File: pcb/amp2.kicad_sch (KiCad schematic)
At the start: 25 parts, among them Q3 BFP640, Q4 BFP640

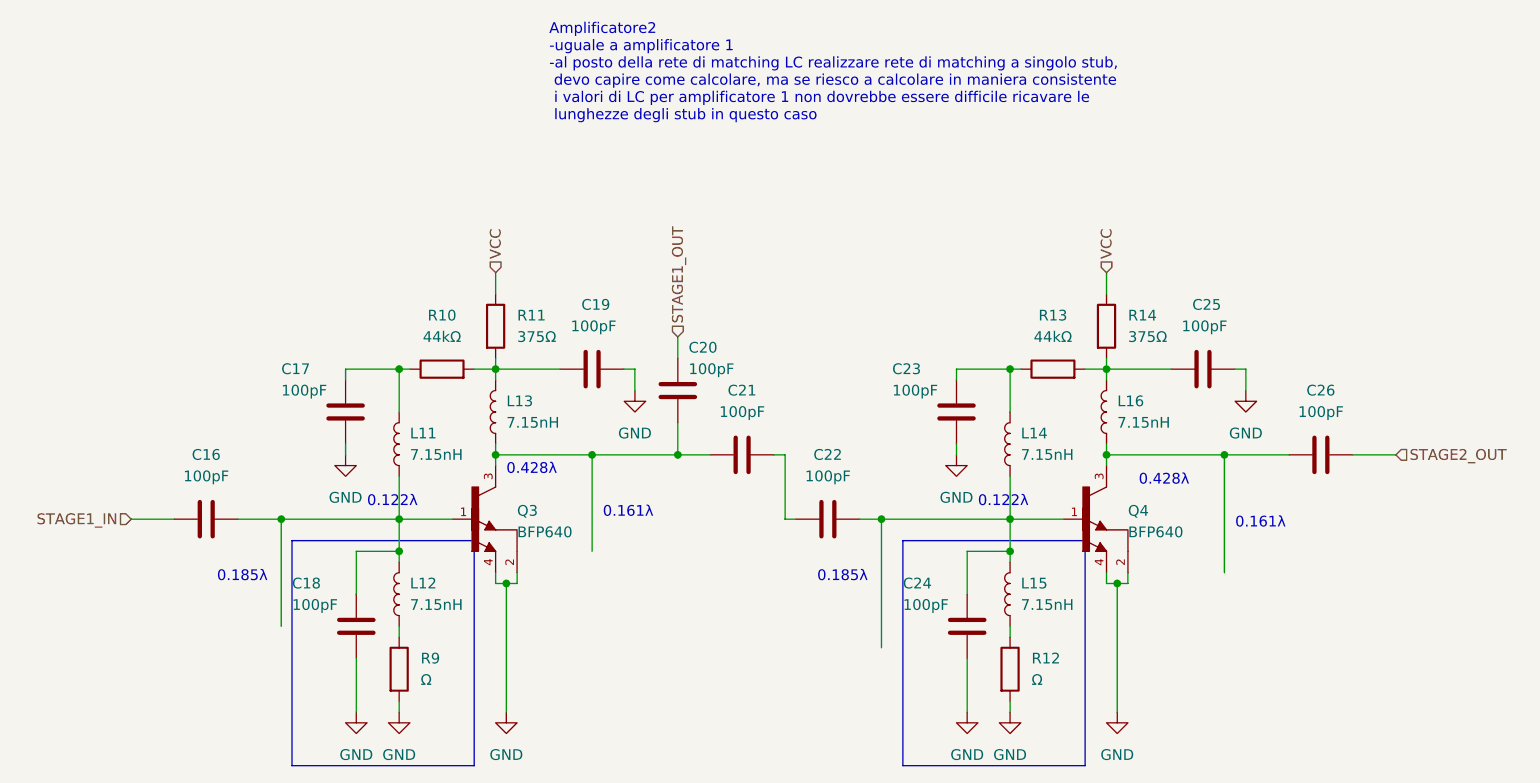
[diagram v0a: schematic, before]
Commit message: Schematic modified as discussed
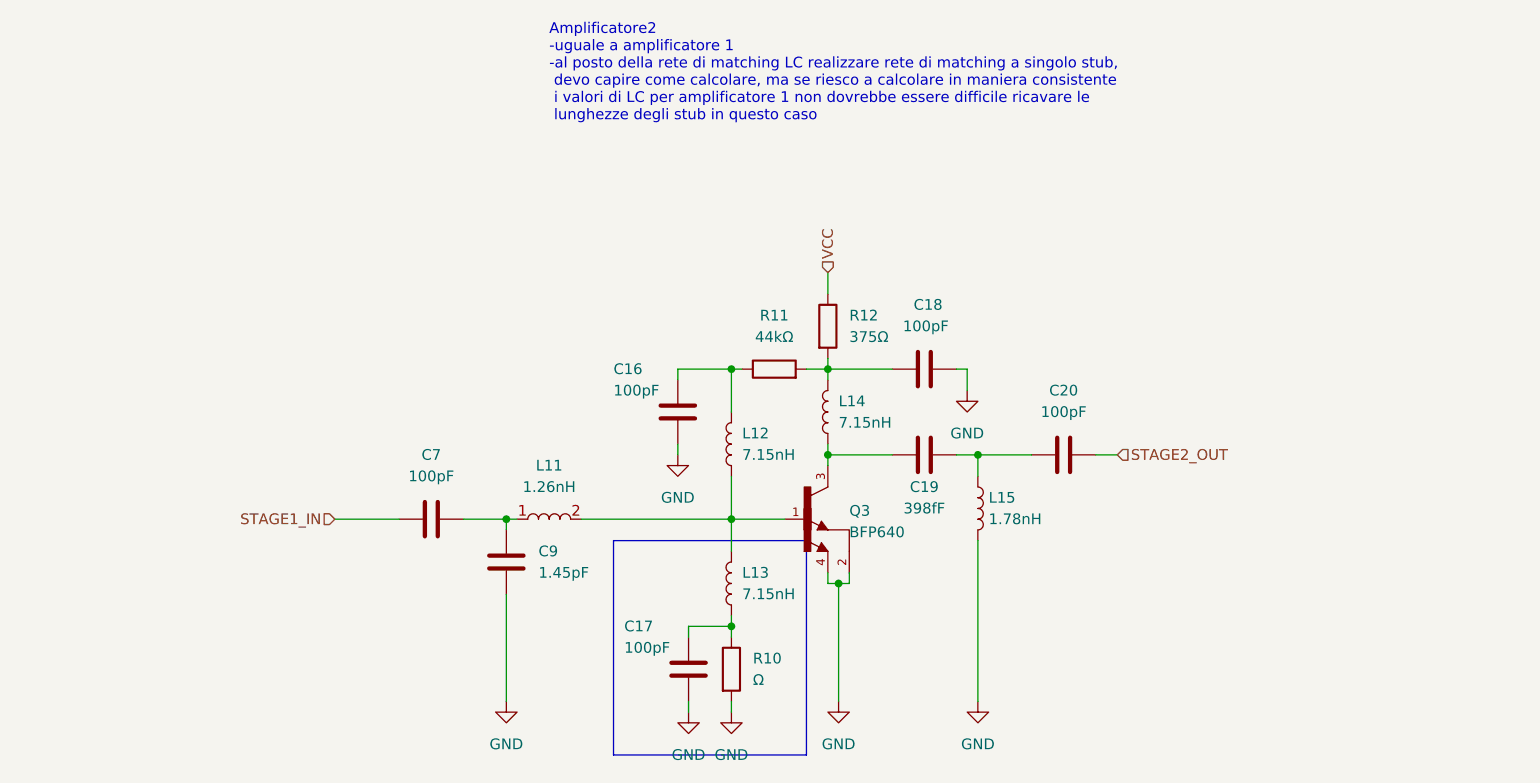
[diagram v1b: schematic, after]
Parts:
- removed C21, C22, C23, C24, C25, C26: 100pF, symbol Device:C
- removed L16: 7.15nH, symbol Device:L
- removed Q4: BFP640, Nicobigio01:SOT-343, symbol Nicobigio01_Transistor_HBT:BFP640
- removed R13: 44kΩ, symbol Device:R
- removed R14: 375Ω, symbol Device:R
- removed R9: Ω, symbol Device:R
- added C7: 100pF, Capacitor_SMD:C_0603_1608Metric, symbol Device:C
- added C9: 1.45pF, Capacitor_SMD:C_0603_1608Metric, symbol Device:C
- C16, C17, C18, C20: footprint (none) -> Capacitor_SMD:C_0603_1608Metric
- C19: value 100pF -> 398fF; footprint (none) -> Capacitor_SMD:C_0603_1608Metric
- L11: value 7.15nH -> 1.26nH; footprint (none) -> Nicobigio01:Coilcraft_0906-xxLx
- L12, L13, L14: footprint (none) -> Nicobigio01:Coilcraft_1606-xxLx
- L15: value 7.15nH -> 1.78nH; footprint (none) -> Nicobigio01:Coilcraft_0906-xxLx
- R10: value 44kΩ -> Ω; footprint (none) -> Resistor_SMD:R_0603_1608Metric
- R11: value 375Ω -> 44kΩ; footprint (none) -> Resistor_SMD:R_0603_1608Metric
- R12: value Ω -> 375Ω; footprint (none) -> Resistor_SMD:R_0603_1608Metric
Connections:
- net STAGE1_OUT is gone; now on an unnamed net: C20.1
- net GND: now also C16.2, L15.2, R10.2, C9.2; no longer C19.2, R12.2
- net STAGE1_IN: now also C7.1; no longer C16.1
- net STAGE2_OUT: now also C20.2
- net VCC: now also R12.1; no longer R11.1
- net at L14.2: now also C18.1, R11.2, R12.2
- net at L14.1: now also C19.1, Q3.3; no longer L15.2
- net at C17.1, R10.1: now also L13.1; no longer L11.2
- net at L15.1: now also C19.2; no longer R12.1
- net at L12.1: now also L11.2, L13.2, Q3.1
- new net: C7.2, C9.1, L11.1
- new net: C16.1, L12.2, R11.1
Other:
- note removed: "0.122λ"
- note removed: "0.161λ"
- note removed: "0.185λ"
- note removed: "0.428λ"
